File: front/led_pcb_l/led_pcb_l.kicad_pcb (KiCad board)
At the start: 2 copper layers, 5 x 23.2 mm, 4 parts

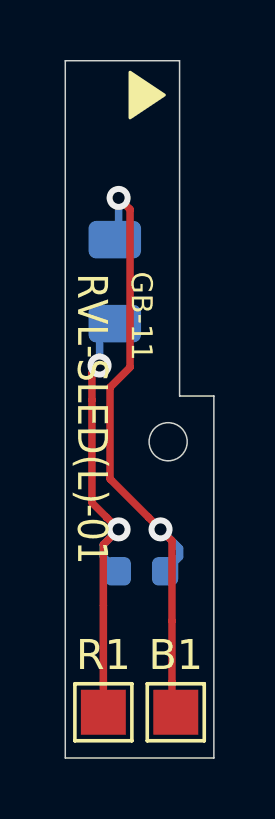
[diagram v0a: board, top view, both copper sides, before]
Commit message: adjust left pcb
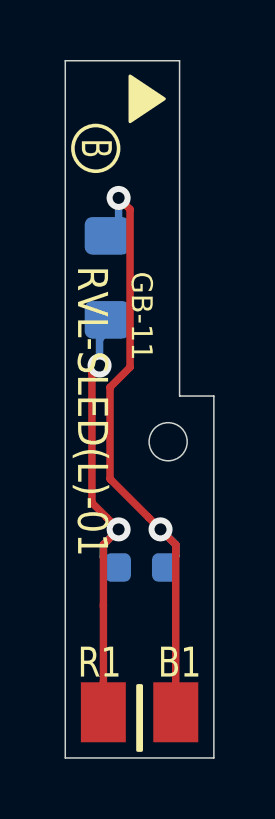
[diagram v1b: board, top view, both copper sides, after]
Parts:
- moved D1 0.28 mm to (45.7, 31.6), turned to 90 degrees
- moved D3 0.13 mm to (46.9, 41.3), turned to 180 degrees
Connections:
- B1 pad 1: Net-(B1_1-Pad1) -> Net-(B1-Pad1)
- D1 pad 1: Net-(B1_1-Pad1) -> Net-(D1-Pad1)
- D1 pad 2: Net-(D1-Pad2) -> Net-(B1-Pad1)
- D3 pad 1: Net-(D1-Pad2) -> Net-(B1-Pad1)
- D3 pad 2: Net-(B1_1-Pad1) -> Net-(D1-Pad1)
- R1 pad 1: Net-(D1-Pad2) -> Net-(D1-Pad1)
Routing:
- net Net-(B1_1-Pad1): track 21.7 -> 0.00 mm, vias 2 -> 0
- net Net-(B1-Pad1): track 0.00 -> 21.7 mm, vias 0 -> 2
- net Net-(D1-Pad2): track 15.7 -> 0.00 mm, vias 2 -> 0
- net Net-(D1-Pad1): track 0.00 -> 15.7 mm, vias 0 -> 2
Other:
- board text added: "A"
- board text added: "B"
- board text added: "B-19"
- board text added: "CG"
- board text added: "Side"
